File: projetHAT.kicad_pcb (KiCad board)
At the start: 2 copper layers, 11 parts, among them J1 Raspberry_Pi_2_3, U1 MCP23S17-E_SO, U2 ULN2803A, U3 AT24CS32-SSHM

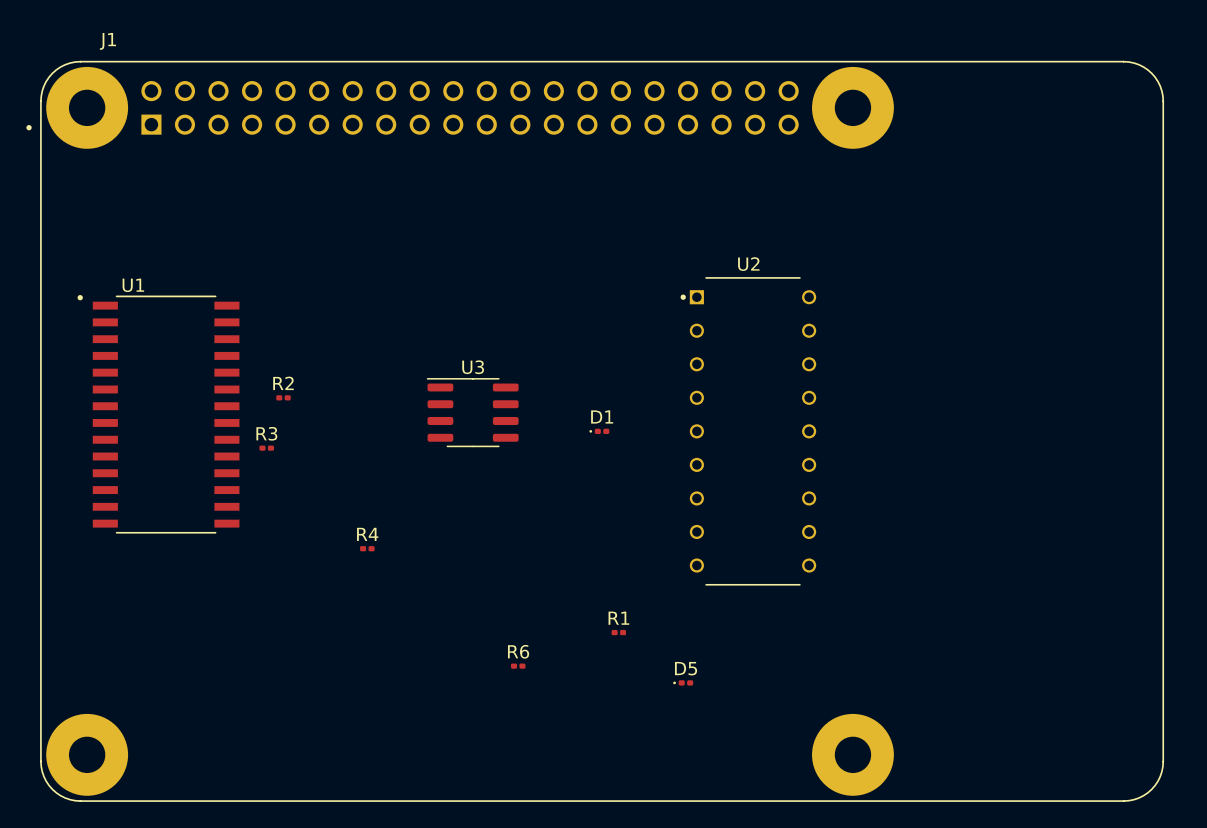
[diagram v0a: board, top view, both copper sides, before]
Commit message: Add files via upload
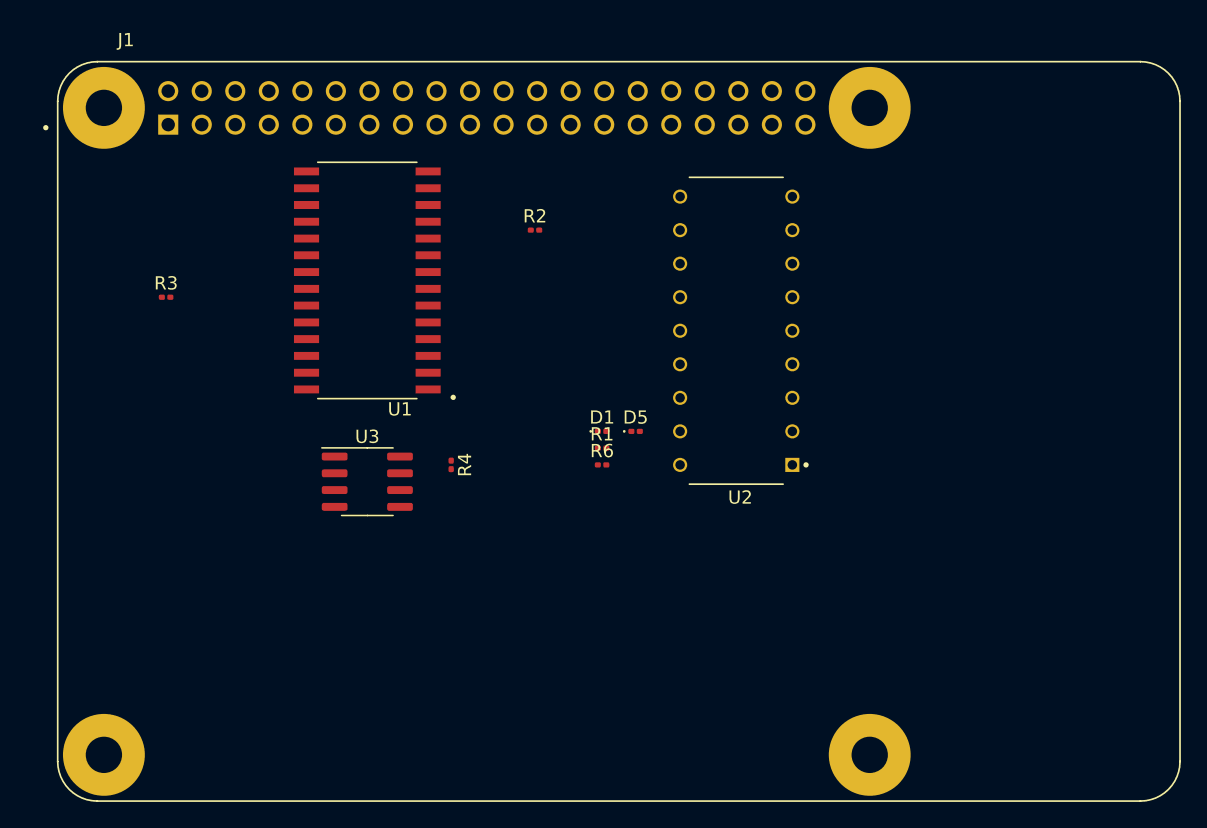
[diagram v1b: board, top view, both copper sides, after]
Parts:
- moved R2 22.9 mm to (73.7, 76.2)
- moved D5 19.4 mm to (81.3, 91.4)
- moved U1 18.3 mm to (61.0, 80.0), turned to 180 degrees
- moved R6 16.5 mm to (78.7, 94.0)
- moved R1 14.0 mm to (78.7, 92.7)
- moved R3 13.7 mm to (45.7, 81.3)
- moved U3 9.57 mm to (61.0, 95.2)
- moved R4 8.98 mm to (67.3, 94.0), turned to 270 degrees
- moved U2 7.73 mm to (88.9, 83.8), turned to 180 degrees
- moved J1 1.27 mm to (80.0, 91.4)
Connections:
- R1 pad 2: Net-(D5-Pad1) -> Net-(D1-Pad2)
- R6 pad 2: Net-(D1-Pad1) -> Net-(D5-Pad2)
- U1 pad 11: Net-(U1-Pad11) -> Net-(J1-Pad24)
- U1 pad 12: Net-(J1-Pad1) -> Net-(J1-Pad23)
- U1 pad 13: Net-(U1-Pad13) -> Net-(J1-Pad19)
- U1 pad 14: Net-(J1-Pad1) -> Net-(J1-Pad21)
- U1 pad 15: Net-(U1-Pad15) -> GND
- U1 pad 16: Net-(J1-Pad1) -> GND
- U1 pad 17: Net-(J1-Pad1) -> GND
- U1 pad 18: Net-(U1-Pad18) -> Net-(J1-Pad7)
- U1 pad 19: GND -> Net-(U1-Pad19)
- U1 pad 2: GND -> Net-(U1-Pad2)
- U1 pad 21: Net-(J1-Pad24) -> Net-(J1-Pad1)
- U1 pad 22: Net-(J1-Pad7) -> Net-(J1-Pad1)
- U1 pad 23: Net-(J1-Pad23) -> Net-(J1-Pad1)
- U1 pad 25: Net-(J1-Pad19) -> GND
- U1 pad 27: Net-(J1-Pad21) -> GND
- U1 pad 4: GND -> Net-(U1-Pad4)
- U1 pad 6: GND -> Net-(U1-Pad6)
- U1 pad 8: GND -> Net-(U1-Pad8)
- U1 pad 9: Net-(U1-Pad9) -> Net-(J1-Pad1)
- U2 pad 1: Net-(J1-Pad2) -> Net-(U2-Pad1)
- U2 pad 10: Net-(U1-Pad9) -> Net-(J1-Pad2)
- U2 pad 12: Net-(U2-Pad12) -> Net-(D1-Pad1)
- U2 pad 14: Net-(U2-Pad14) -> Net-(D5-Pad1)
- U2 pad 2: GND -> Net-(U2-Pad2)
- U2 pad 5: Net-(D1-Pad2) -> Net-(U1-Pad5)
- U2 pad 6: Net-(U1-Pad13) -> Net-(U2-Pad6)
- U2 pad 7: Net-(D5-Pad2) -> Net-(U1-Pad7)
- U2 pad 9: Net-(U2-Pad9) -> GND
